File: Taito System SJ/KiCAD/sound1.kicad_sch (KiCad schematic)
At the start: 36 parts, among them U26 74LS367, U31 74LS393, U38 74LS374, U40 74LS393, U41 74LS08, U44 74LS74, U45 74LS74, U46 74LS74, U48 74LS367, U52 Z80-A (SOUND CPU), U54 74LS32, U58 74LS04, U59 74LS138, U61 NEC_UPD2114, U62 NEC_UPD2114, U64 74LS74, U70-ROM1 M2732, U71-ROM2 M2732, U72-ROM3 M2732, U73-ROM4 M2732, U94 74LS04

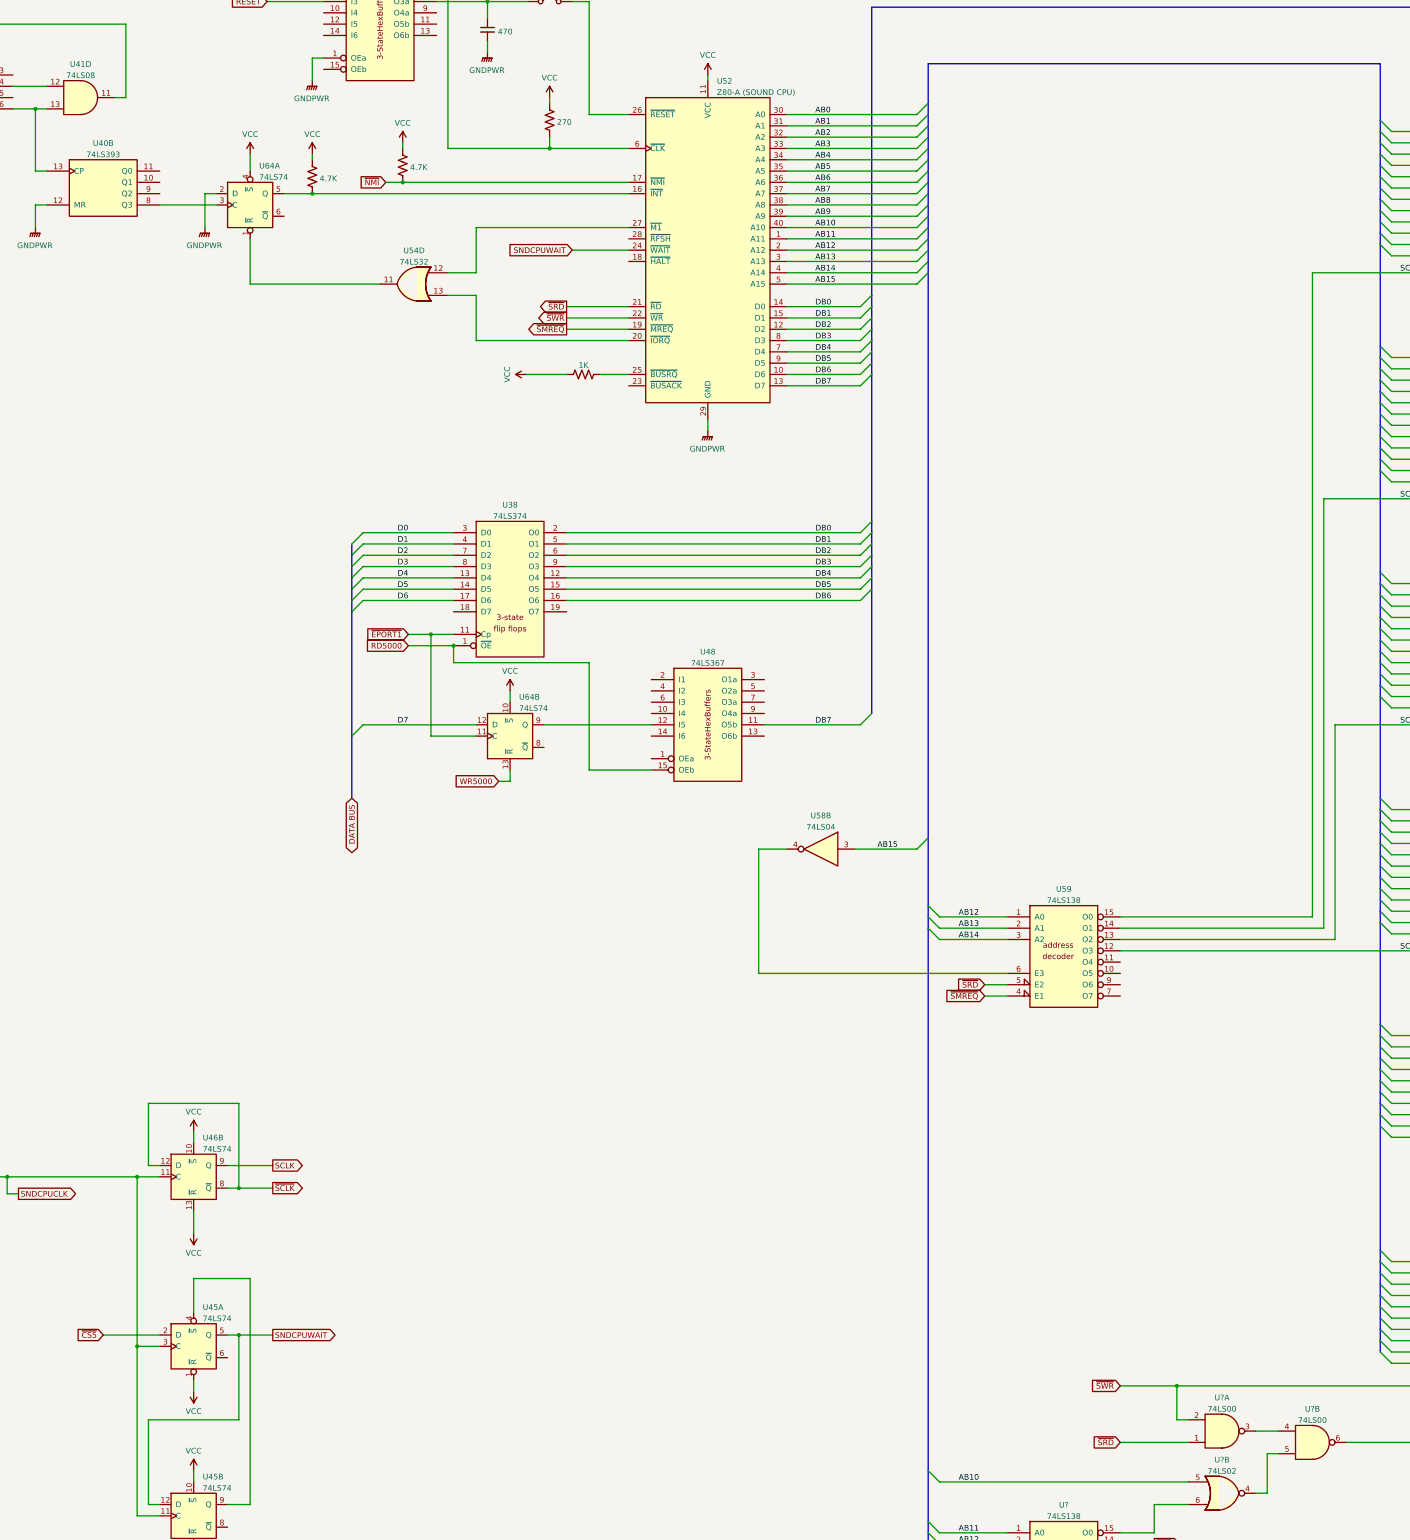
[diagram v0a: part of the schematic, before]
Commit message: Update before transfer
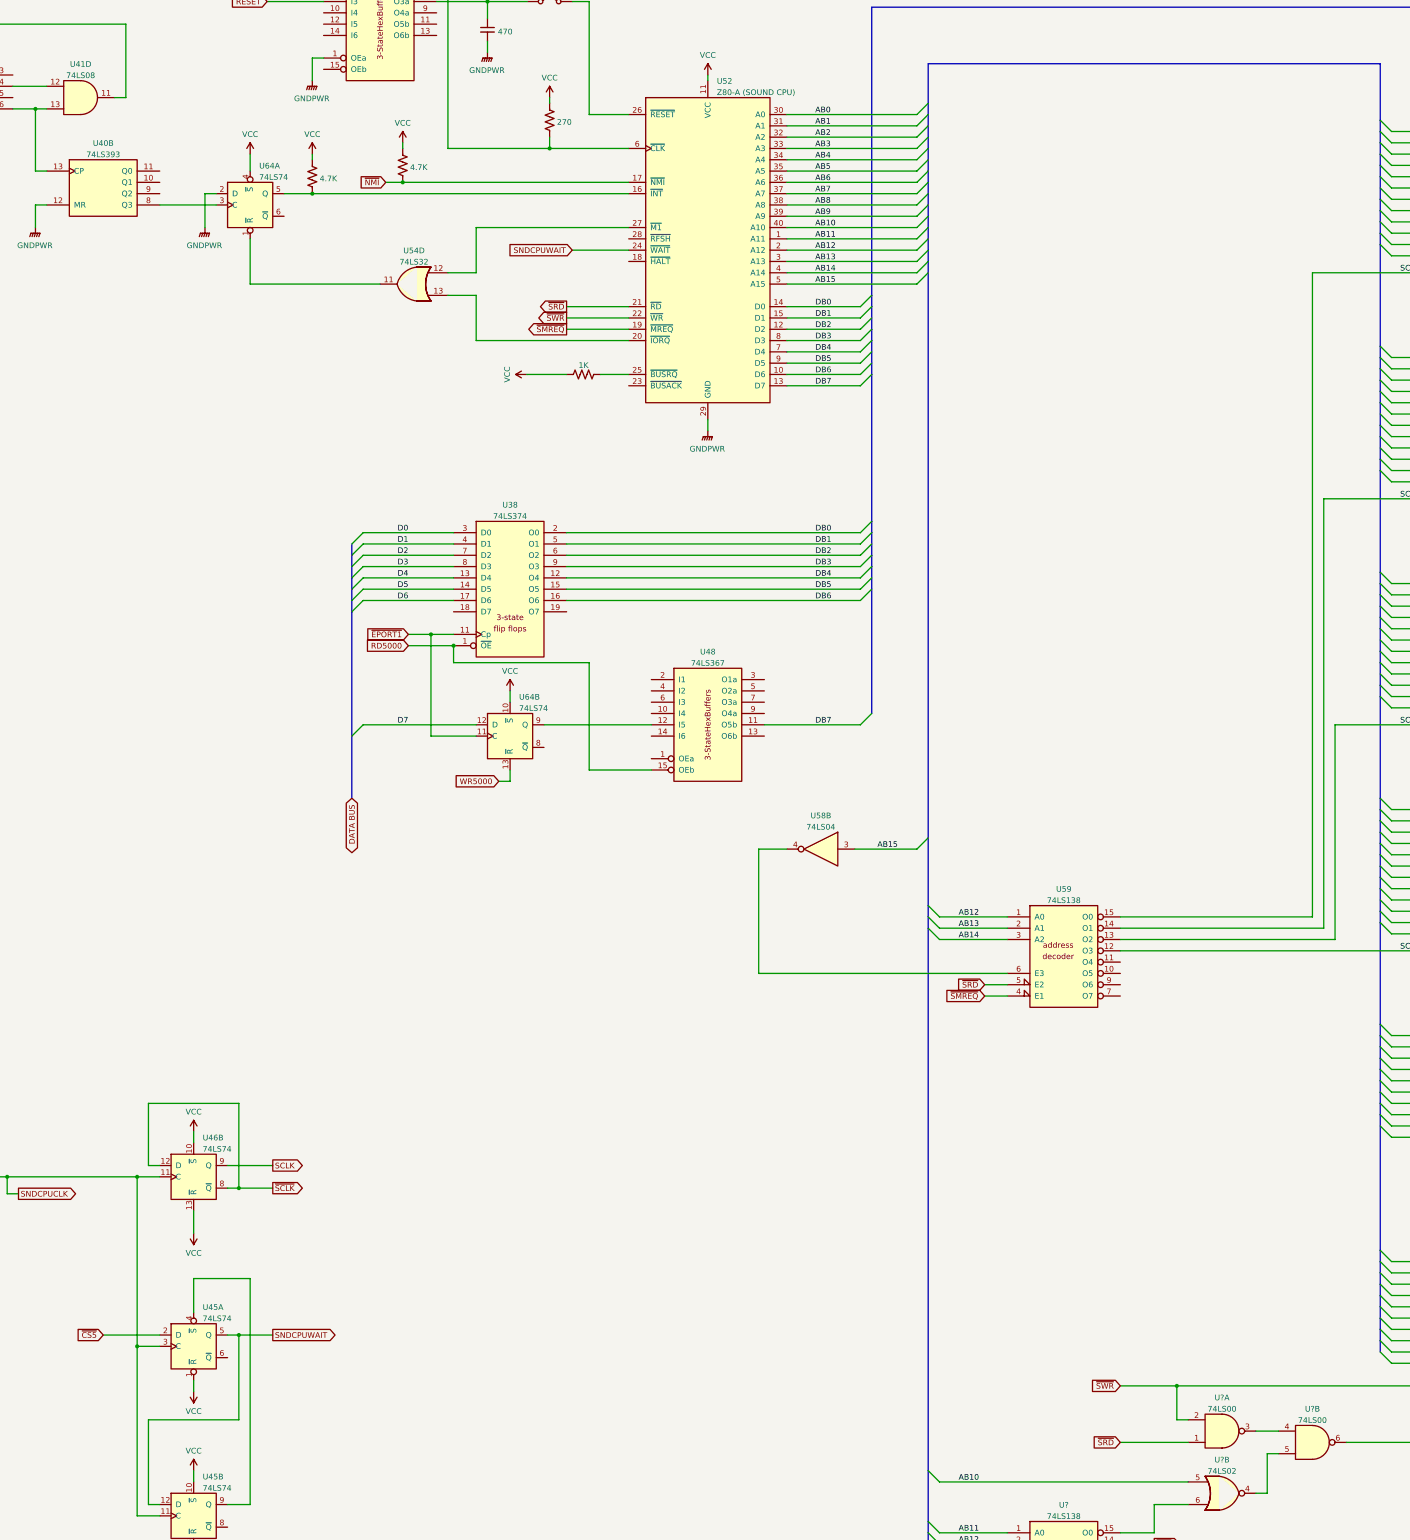
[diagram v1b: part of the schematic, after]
